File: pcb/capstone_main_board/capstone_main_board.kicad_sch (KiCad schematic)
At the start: 46 parts, among them J1 Vin, J10 MOSI, J11 SCLK, J12 NCS, J13 Vin, J18 SDO, J19 BAT, J2 VDD OS, J20 IO14, J21 IO13, J22 IO10, J23 IO8, J24 IO6, J25 RX0, J26 TX0, J27 D+, J28 D-, J29 100, J3 VDDA, J30 5V, J31 RESET, J32 Vin, J4 MFIO, J5 VDD FS, J6 V2, J7 V1, J8 Motion, J9 MISO, Q1 BSS138, Q2 BSS138, U1 OMGS3, U2 ADXL345, U3 TPS73219DBVT, U5 VREG_SOT23-5

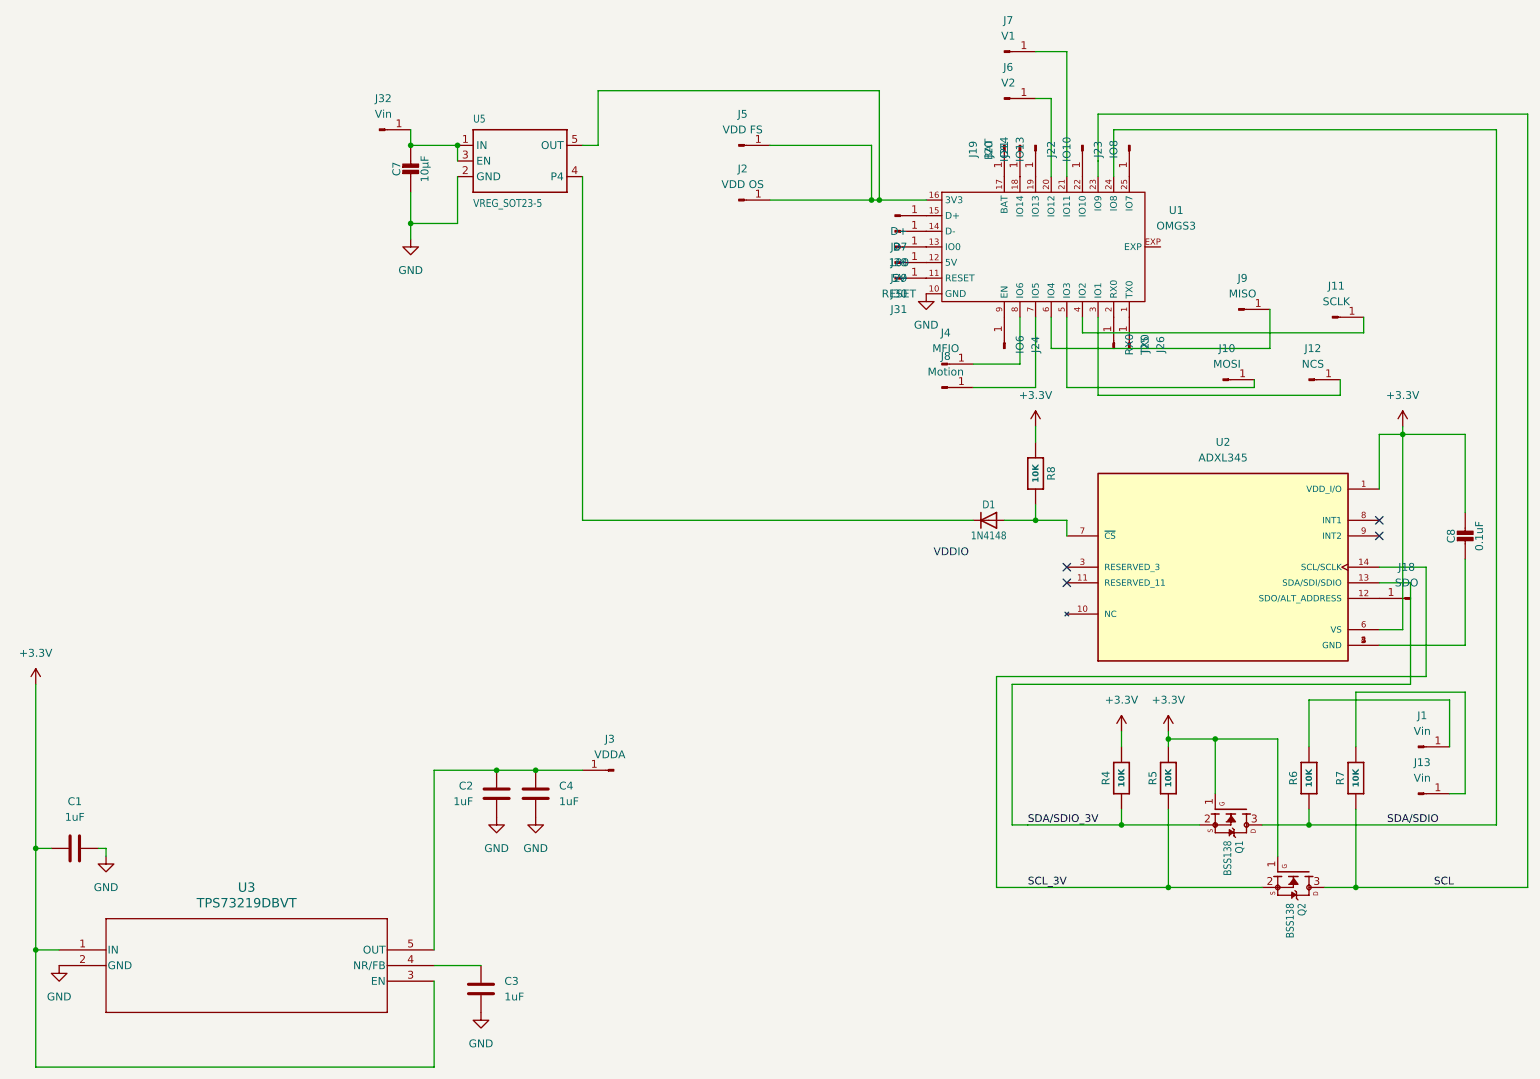
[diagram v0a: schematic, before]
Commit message: sensor and mcu board nearly complete
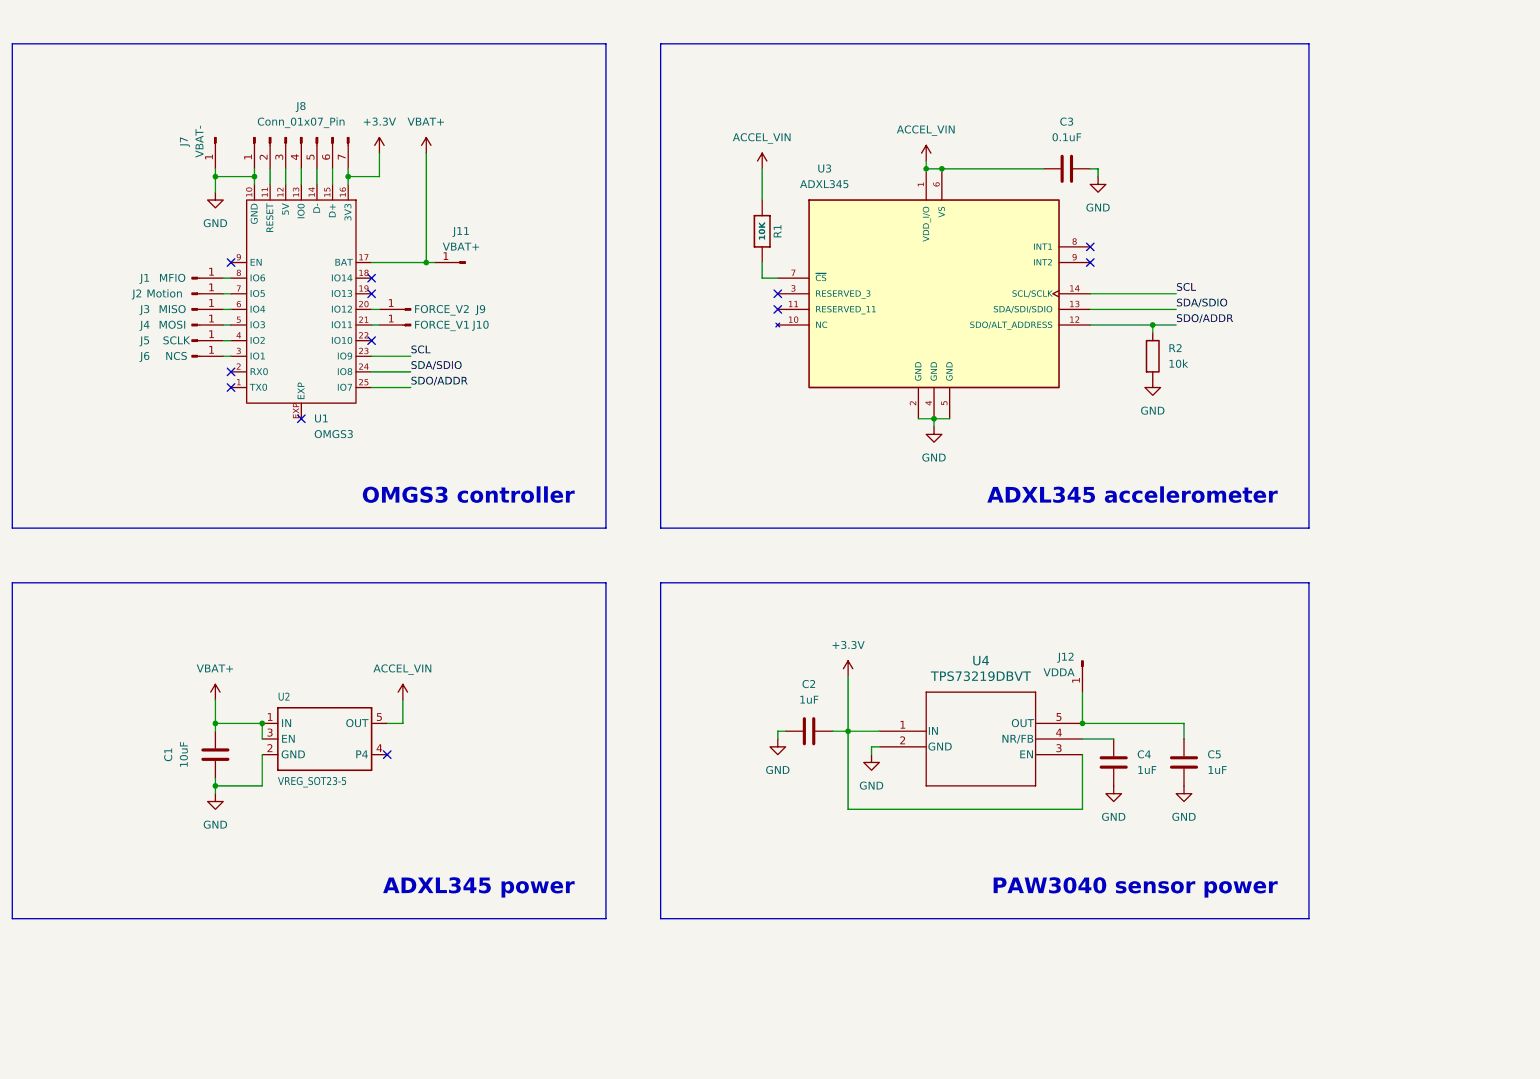
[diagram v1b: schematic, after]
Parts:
- removed C2, C4: 1uF, Library:CAP_CL10_SAM, symbol Device:C
- removed C7: 10µF, Library:CAP_CL21_SAM, symbol Adafruit ADXL345 Triple-Axis Accelerometer-eagle-import:CAP_CERAMIC0805-NOOUTLI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
- removed C8: 0.1uF, Library:CAP_CL05_SAM, symbol Adafruit ADXL345 Triple-Axis Accelerometer-eagle-import:CAP_CERAMIC0805-NOOUTLI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
- removed D1: 1N4148, Library:SOD3715X135N, symbol Adafruit ADXL345 Triple-Axis Accelerometer-eagle-import:microbuilder_DIODE_SOD3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
- removed J1, J13, J32: Vin, Connector_PinHeader_1.00mm:PinHeader_1x01_P1.00mm_Vertical, symbol Connector:Conn_01x01_Pin
- removed J18: SDO, Connector_PinHeader_1.00mm:PinHeader_1x01_P1.00mm_Vertical, symbol Connector:Conn_01x01_Pin
- removed J2: VDD OS, Connector_PinHeader_1.00mm:PinHeader_1x01_P1.00mm_Vertical, symbol Connector:Conn_01x01_Pin
- removed J20: IO14, Connector_PinHeader_1.00mm:PinHeader_1x01_P1.00mm_Vertical, symbol Connector:Conn_01x01_Pin
- removed J21: IO13, Connector_PinHeader_1.00mm:PinHeader_1x01_P1.00mm_Vertical, symbol Connector:Conn_01x01_Pin
- removed J22: IO10, Connector_PinHeader_1.00mm:PinHeader_1x01_P1.00mm_Vertical, symbol Connector:Conn_01x01_Pin
- removed J23: IO8, Connector_PinHeader_1.00mm:PinHeader_1x01_P1.00mm_Vertical, symbol Connector:Conn_01x01_Pin
- removed J24: IO6, Connector_PinHeader_1.00mm:PinHeader_1x01_P1.00mm_Vertical, symbol Connector:Conn_01x01_Pin
- removed J25: RX0, Connector_PinHeader_1.00mm:PinHeader_1x01_P1.00mm_Vertical, symbol Connector:Conn_01x01_Pin
- removed J26: TX0, Connector_PinHeader_1.00mm:PinHeader_1x01_P1.00mm_Vertical, symbol Connector:Conn_01x01_Pin
- removed J27: D+, Connector_PinHeader_1.00mm:PinHeader_1x01_P1.00mm_Vertical, symbol Connector:Conn_01x01_Pin
- removed J28: D-, Connector_PinHeader_1.00mm:PinHeader_1x01_P1.00mm_Vertical, symbol Connector:Conn_01x01_Pin
- removed J29: 100, Connector_PinHeader_1.00mm:PinHeader_1x01_P1.00mm_Vertical, symbol Connector:Conn_01x01_Pin
- removed J30: 5V, Connector_PinHeader_1.00mm:PinHeader_1x01_P1.00mm_Vertical, symbol Connector:Conn_01x01_Pin
- removed J31: RESET, Connector_PinHeader_1.00mm:PinHeader_1x01_P1.00mm_Vertical, symbol Connector:Conn_01x01_Pin
- removed J5: VDD FS, Connector_PinHeader_1.00mm:PinHeader_1x01_P1.00mm_Vertical, symbol Connector:Conn_01x01_Pin
- removed Q1, Q2: BSS138, Library:SOT95P240X111-3N, symbol Adafruit ADXL345 Triple-Axis Accelerometer-eagle-import:MOSFET-NWIDE
- removed R4, R5, R6, R7: 10K, Library:RES_ERJ2RKF1002X, symbol Adafruit ADXL345 Triple-Axis Accelerometer-eagle-import:RESISTOR0805_NOOUTLINE
- removed U1: OMGS3, Library:OMGS3, symbol New_Library:OMGS3
- removed U2: ADXL345, Library:PQFN80P500X300X100-14N, symbol New_Library:ADXL345
- removed U3: TPS73219DBVT, Library:DBV5_TEX, symbol New_Library:TPS73219DBVT
- added C1: 10uF, Capacitor_SMD:C_0805_2012Metric, symbol Device:C
- added C3: 0.1uF, Capacitor_SMD:C_0402_1005Metric, symbol Device:C
- added C5: 1uF, Capacitor_SMD:C_0603_1608Metric, symbol Device:C
- added J7: VBAT-, Connector_PinHeader_2.00mm:PinHeader_1x01_P2.00mm_Vertical, symbol Connector:Conn_01x01_Pin
- added J8: Conn_01x07_Pin, Custom_FP:OMGS3_programming_pins, symbol Connector:Conn_01x07_Pin
- added R2: 10k, Resistor_SMD:R_0402_1005Metric, symbol Device:R
- added U1: OMGS3, Imported_FP:OMGS3, symbol Imported_sym:OMGS3
- added U3: ADXL345, Imported_FP:PQFN80P500X300X100-14N, symbol Imported_sym:ADXL345
- added U4: TPS73219DBVT, Imported_FP:DBV5_TEX, symbol Custom_sym:TPS73219DBVT
- C2: renamed from C1; footprint Library:CAP_CL10_SAM -> Capacitor_SMD:C_0603_1608Metric
- C4: renamed from C3; footprint Library:CAP_CL10_SAM -> Capacitor_SMD:C_0603_1608Metric
- J1: renamed from J4; footprint Connector_PinHeader_1.00mm:PinHeader_1x01_P1.00mm_Vertical -> Connector_PinHeader_2.00mm:PinHeader_1x01_P2.00mm_Vertical
- J10: renamed from J7; value V1 -> FORCE_V1; footprint Connector_PinHeader_1.00mm:PinHeader_1x01_P1.00mm_Vertical -> Connector_PinHeader_2.00mm:PinHeader_1x01_P2.00mm_Vertical
- J11: renamed from J19; value BAT -> VBAT+; footprint Connector_PinHeader_1.00mm:PinHeader_1x01_P1.00mm_Vertical -> Connector_PinHeader_2.00mm:PinHeader_1x01_P2.00mm_Vertical
- J12: renamed from J3; footprint Connector_PinHeader_1.00mm:PinHeader_1x01_P1.00mm_Vertical -> Connector_PinHeader_2.00mm:PinHeader_1x01_P2.00mm_Vertical
- J2: renamed from J8; footprint Connector_PinHeader_1.00mm:PinHeader_1x01_P1.00mm_Vertical -> Connector_PinHeader_2.00mm:PinHeader_1x01_P2.00mm_Vertical
- J3: renamed from J9; footprint Connector_PinHeader_1.00mm:PinHeader_1x01_P1.00mm_Vertical -> Connector_PinHeader_2.00mm:PinHeader_1x01_P2.00mm_Vertical
- J4: renamed from J10; footprint Connector_PinHeader_1.00mm:PinHeader_1x01_P1.00mm_Vertical -> Connector_PinHeader_2.00mm:PinHeader_1x01_P2.00mm_Vertical
- J5: renamed from J11; footprint Connector_PinHeader_1.00mm:PinHeader_1x01_P1.00mm_Vertical -> Connector_PinHeader_2.00mm:PinHeader_1x01_P2.00mm_Vertical
- J6: renamed from J12; footprint Connector_PinHeader_1.00mm:PinHeader_1x01_P1.00mm_Vertical -> Connector_PinHeader_2.00mm:PinHeader_1x01_P2.00mm_Vertical
- J9: renamed from J6; value V2 -> FORCE_V2; footprint Connector_PinHeader_1.00mm:PinHeader_1x01_P1.00mm_Vertical -> Connector_PinHeader_2.00mm:PinHeader_1x01_P2.00mm_Vertical
- R1: renamed from R8; footprint Library:RES_ERJ2RKF1002X -> Resistor_SMD:R_0402_1005Metric
- U2: renamed from U5; footprint Library:SOT95P285X140-5N -> Imported_FP:SOT95P280X145-5N
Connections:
- net +3.3V: now also C2.1, J8.7 (Pin_7), U1.16 (3V3), U4.1 (IN), U4.3 (EN); no longer C2.2, R1.2
- net GND: now also C2.2, C1.1, C3.1, C5.2, J7.1 (Pin_1), J8.1 (Pin_1), R2.2, U1.10 (GND), U3.2 (GND), U3.4 (GND), U3.5 (GND), U4.2 (GND); no longer C2.1
- net SCL: now also U1.23 (IO9), U3.14 (SCL/SCLK)
- net SDA/SDIO: now also U1.24 (IO8), U3.13 (SDA/SDI/SDIO)
- net ACCEL_VIN: now reaches U2.5 (OUT)
- net ACCEL_VIN: now also R1.2, C3.2, U3.1 (VDD_I/O), U3.6 (VS)
- net VBAT+: now reaches U2.1 (IN), U2.3 (EN)
- net VBAT+: now also J11.1 (Pin_1), C1.2, U1.17 (BAT)
- net at C4.1: now also U4.4 (NR/FB)
- net at J12.1 (Pin_1): now also C5.1, U4.5 (OUT)
- net at J1.1 (Pin_1): now also U1.8 (IO6)
- net at J3.1 (Pin_1): now also U1.6 (IO4)
- net at R1.1: now also U3.7 (~{CS})
- net at J9.1 (Pin_1): now also U1.20 (IO12)
- net at J10.1 (Pin_1): now also U1.21 (IO11)
- net at J6.1 (Pin_1): now also U1.3 (IO1)
- net at J5.1 (Pin_1): now also U1.4 (IO2)
- net at J4.1 (Pin_1): now also U1.5 (IO3)
- net at J2.1 (Pin_1): now also U1.7 (IO5)
- new net: J8.2 (Pin_2), U1.11 (RESET)
- new net: J8.3 (Pin_3), U1.12 (5V)
- new net: J8.4 (Pin_4), U1.13 (IO0)
- new net: J8.5 (Pin_5), U1.14 (D-)
- new net: J8.6 (Pin_6), U1.15 (D+)
- new net SDO/ADDR: R2.1, U1.25 (IO7), U3.12 (SDO/ALT_ADDRESS)
- no-connect marks 4 -> 12
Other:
- note added: "ADXL345 accelerometer"
- note added: "ADXL345 power"
- note added: "OMGS3 controller"
- note added: "PAW3040 sensor power"
- note removed: "VDDIO"
- moved on the sheet: C2, C4, J1, J10, J11, J12, J2, J3, J4, J5, J6, J9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
